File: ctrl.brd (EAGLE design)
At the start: 58 x 58 mm, 47 parts, among them U1 TPS92513, U2 TPS92513

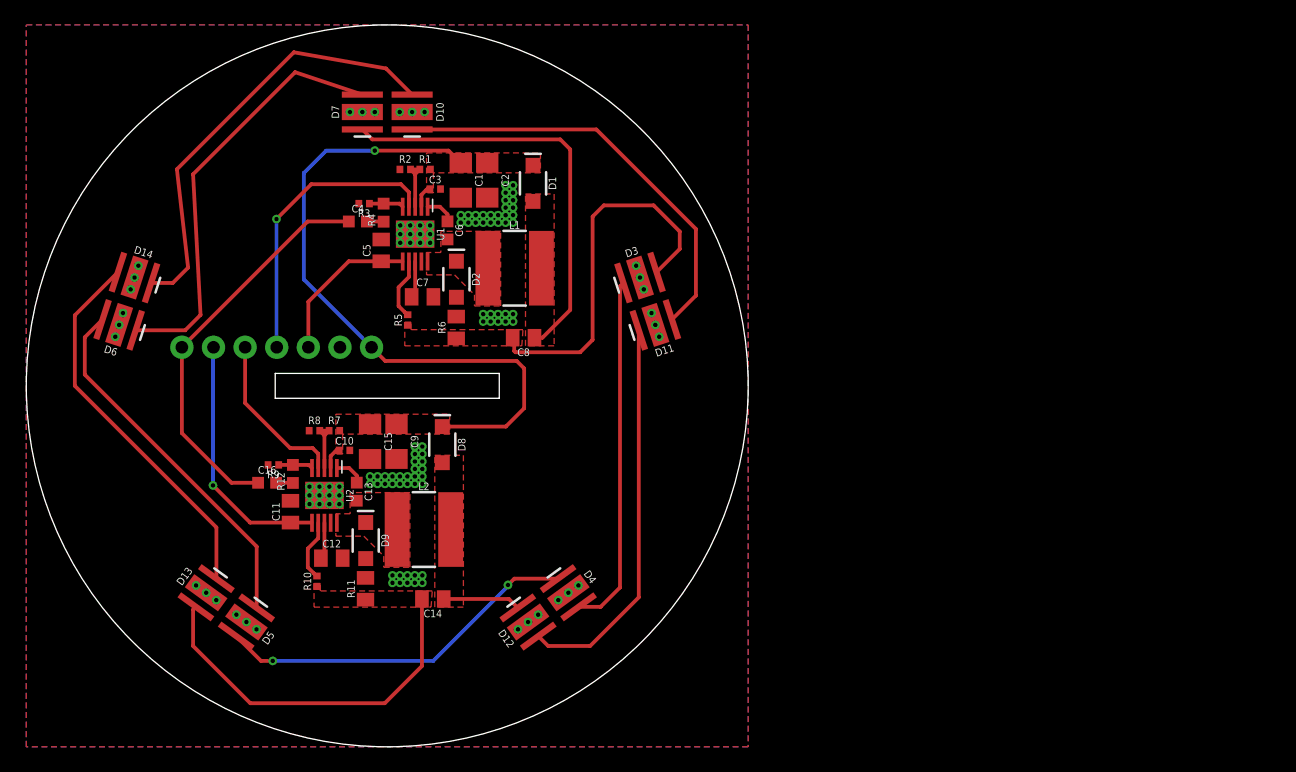
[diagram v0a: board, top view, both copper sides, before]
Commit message: save
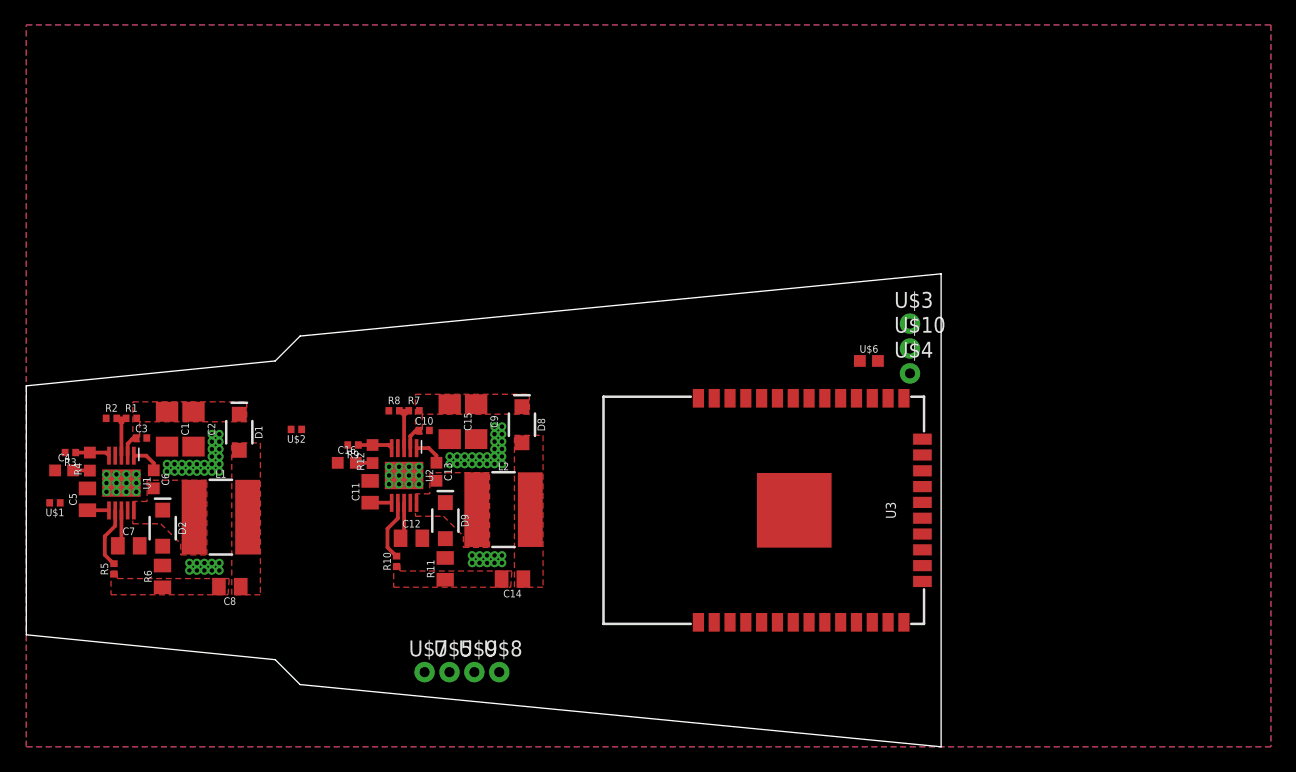
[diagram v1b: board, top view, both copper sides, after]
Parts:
- removed D10, D11, D12, D13, D14, D3, D4, D5, D6, D7: XPGWHT-L1-0000-00BE8, derek:XLAMP-XPG
- removed J45: (no value), derek:1X07_NO_SILK
- added U$1, U$2: 10M, derek:0402
- added U$10, U$3, U$4, U$5, U$7, U$8, U$9: TP-1502, derek:TP-1502
- added U$6: 10k, derek:0603
- added U3: ESP-WROOM-32, derek:ESP-WROOM-32
- moved C2 30.9 mm to (13.4, 25.5)
- moved C4 30.9 mm to (3.04, 22.2)
- moved C5 30.9 mm to (4.91, 19.9)
- moved C6 30.9 mm to (10.2, 21.5)
- moved C7 30.9 mm to (8.23, 16.1)
- moved C8 30.9 mm to (16.4, 12.9)
- moved D2 30.9 mm to (11.0, 17.6)
- moved L1 30.9 mm to (15.6, 18.4)
- moved R2 30.9 mm to (6.84, 26.4)
- moved R3 30.9 mm to (3.54, 23.6)
- moved R4 30.9 mm to (5.11, 22.9)
- moved R5 30.9 mm to (7.04, 14.3)
- moved C1 30.9 mm to (11.3, 25.5)
- moved C3 30.9 mm to (9.25, 24.8)
- moved D1 30.9 mm to (17.1, 25.3)
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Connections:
- removed net N$12: D6.C, D7.A
- removed net N$13: D3.C, D4.A
- removed net N$14: D4.C, D5.A
- removed net N$15: D5.C, D6.A
- removed net N$2: D11.C, D12.A
- removed net N$22: D13.C, D14.A
- removed net N$24: D10.A, D14.C
- removed net N$27: D10.C, D11.A
- new net 3.3V: U$3.1, U$6.2, U3.2
- new net N$29: U$6.1, U3.3
- net 24V: now also U$1.2, U$2.2, U$4.1; no longer J45.7
- net CLK: now also U3.10; no longer J45.1
- net GND-ISO: now also U$10.1, U3.1, U3.15, U3.38, U3.GND; no longer D10.GND, D10.P$1, D10.P$2, D10.P$3, D11.GND, D11.P$1, D11.P$2, D11.P$3, D12.GND, D12.P$1, D12.P$2, D12.P$3, D13.GND, D13.P$1, D13.P$2, D13.P$3, D14.GND, D14.P$1, D14.P$2, D14.P$3, D3.GND, D3.P$1, D3.P$2, D3.P$3, D4.GND, D4.P$1, D4.P$2, D4.P$3, D5.GND, D5.P$1, D5.P$2, D5.P$3, D6.GND, D6.P$1, D6.P$2, D6.P$3, D7.GND, D7.P$1, D7.P$2, D7.P$3, J45.6
- net IADJ1: now also U$1.1; no longer J45.5
- net IADJ2: now also U$2.1; no longer J45.2
- net N$23: now also U$8.1; no longer D12.C
- net N$26: now also U$9.1; no longer D13.A
- net N$6: now also U$7.1; no longer D3.A
- net N$7: now also U$5.1; no longer D7.C
- net PDIM1: now also U3.11; no longer J45.4
- net PDIM2: now also U3.12; no longer J45.3
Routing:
- net 24V: track 57.0 -> 3.63 mm, vias 1 -> 0
- net N$24: track 35.2 -> 0.00 mm
- net N$12: track 34.3 -> 0.00 mm
- net N$27: track 34.2 -> 0.00 mm
- net N$7: track 34.1 -> 0.00 mm
- net CLK: track 32.3 -> 0.00 mm
- net N$2: track 31.5 -> 0.00 mm
- net N$22: track 30.8 -> 0.00 mm
- net N$26: track 30.2 -> 0.00 mm
- net N$6: track 30.1 -> 0.00 mm
- net N$14: track 29.5 -> 0.00 mm, vias 2 -> 0
- net N$15: track 29.5 -> 0.00 mm
- net N$13: track 28.6 -> 0.00 mm
- net PDIM1: track 23.5 -> 0.00 mm, vias 1 -> 0
- net IADJ2: track 20.3 -> 1.74 mm, vias 1 -> 0
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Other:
- board size 58 x 58 mm -> 73.5 x 38 mm

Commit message: saveeee
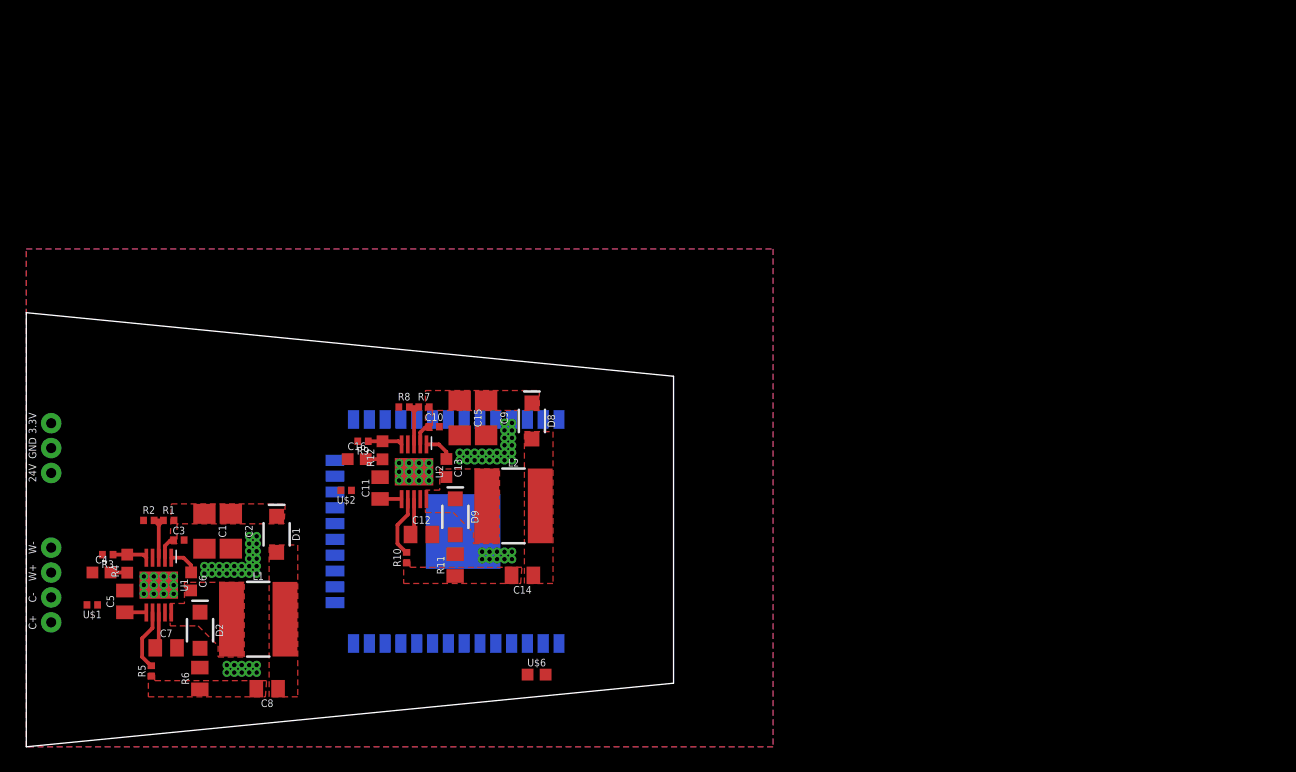
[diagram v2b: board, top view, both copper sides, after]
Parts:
- removed U$10, U$3, U$4, U$5, U$7, U$8, U$9: TP-1502, derek:TP-1502
- added 24V, 3.3V, C+, C-, GND, W+, W-: TP-1502, derek:TP-1502
- moved U$6 36.7 mm to (41.0, 5.80)
- moved U3 26.7 mm to (35.1, 17.3), flipped to the bottom
- moved C2 8.73 mm to (16.4, 17.3)
- moved C3 8.73 mm to (12.3, 16.6)
- moved R4 8.73 mm to (8.11, 14.7)
- moved U1 8.73 mm to (10.6, 13.0)
- moved C1 8.73 mm to (14.3, 17.3)
- moved C4 8.73 mm to (6.04, 14.0)
- moved C5 8.73 mm to (7.91, 11.7)
- moved C6 8.73 mm to (13.2, 13.3)
- moved C7 8.73 mm to (11.2, 7.95)
- moved C8 8.73 mm to (19.4, 4.67)
- moved D1 8.73 mm to (20.1, 17.1)
- moved D2 8.73 mm to (14.0, 9.37)
- moved L1 8.73 mm to (18.6, 10.2)
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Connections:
- net 24V: now also 24V.1; no longer U$4.1
- net 3.3V: now also 3.3V.1; no longer U$3.1
- net GND-ISO: now also GND.1; no longer U$10.1
- net N$23: now also W+.1; no longer U$8.1
- net N$26: now also W-.1; no longer U$9.1
- net N$6: now also C-.1; no longer U$7.1
- net N$7: now also C+.1; no longer U$5.1
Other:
- board size 73.5 x 38 mm -> 52 x 34.9 mm
